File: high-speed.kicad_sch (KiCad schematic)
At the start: 2 parts, among them J301 245863050104829+

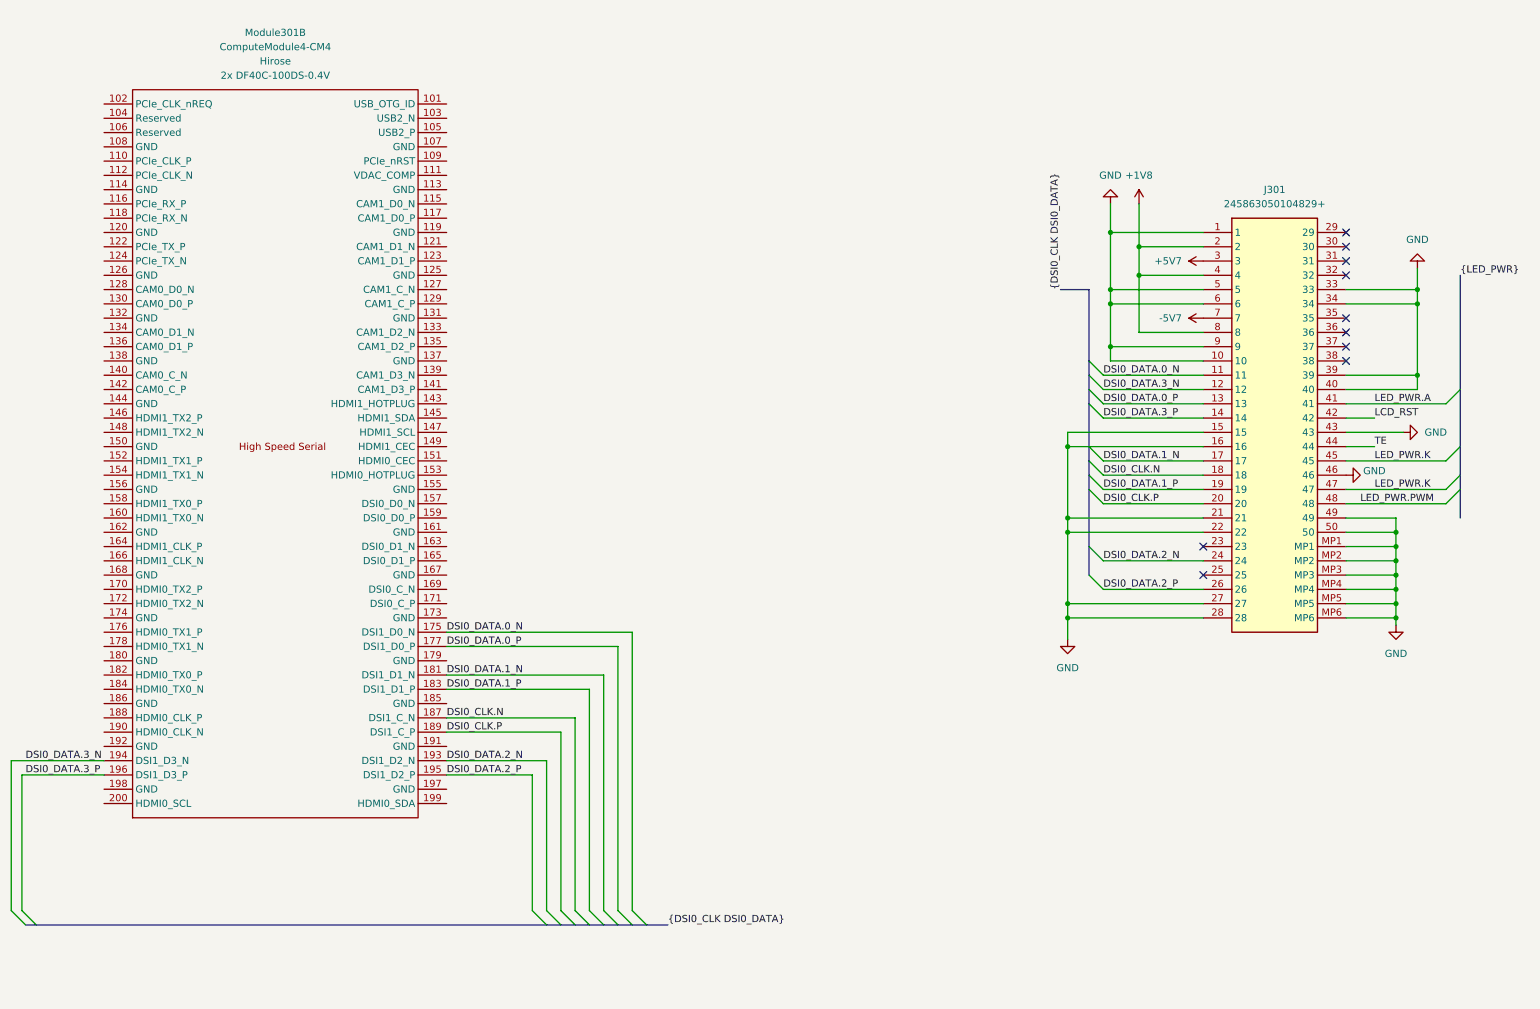
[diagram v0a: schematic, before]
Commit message: more routing
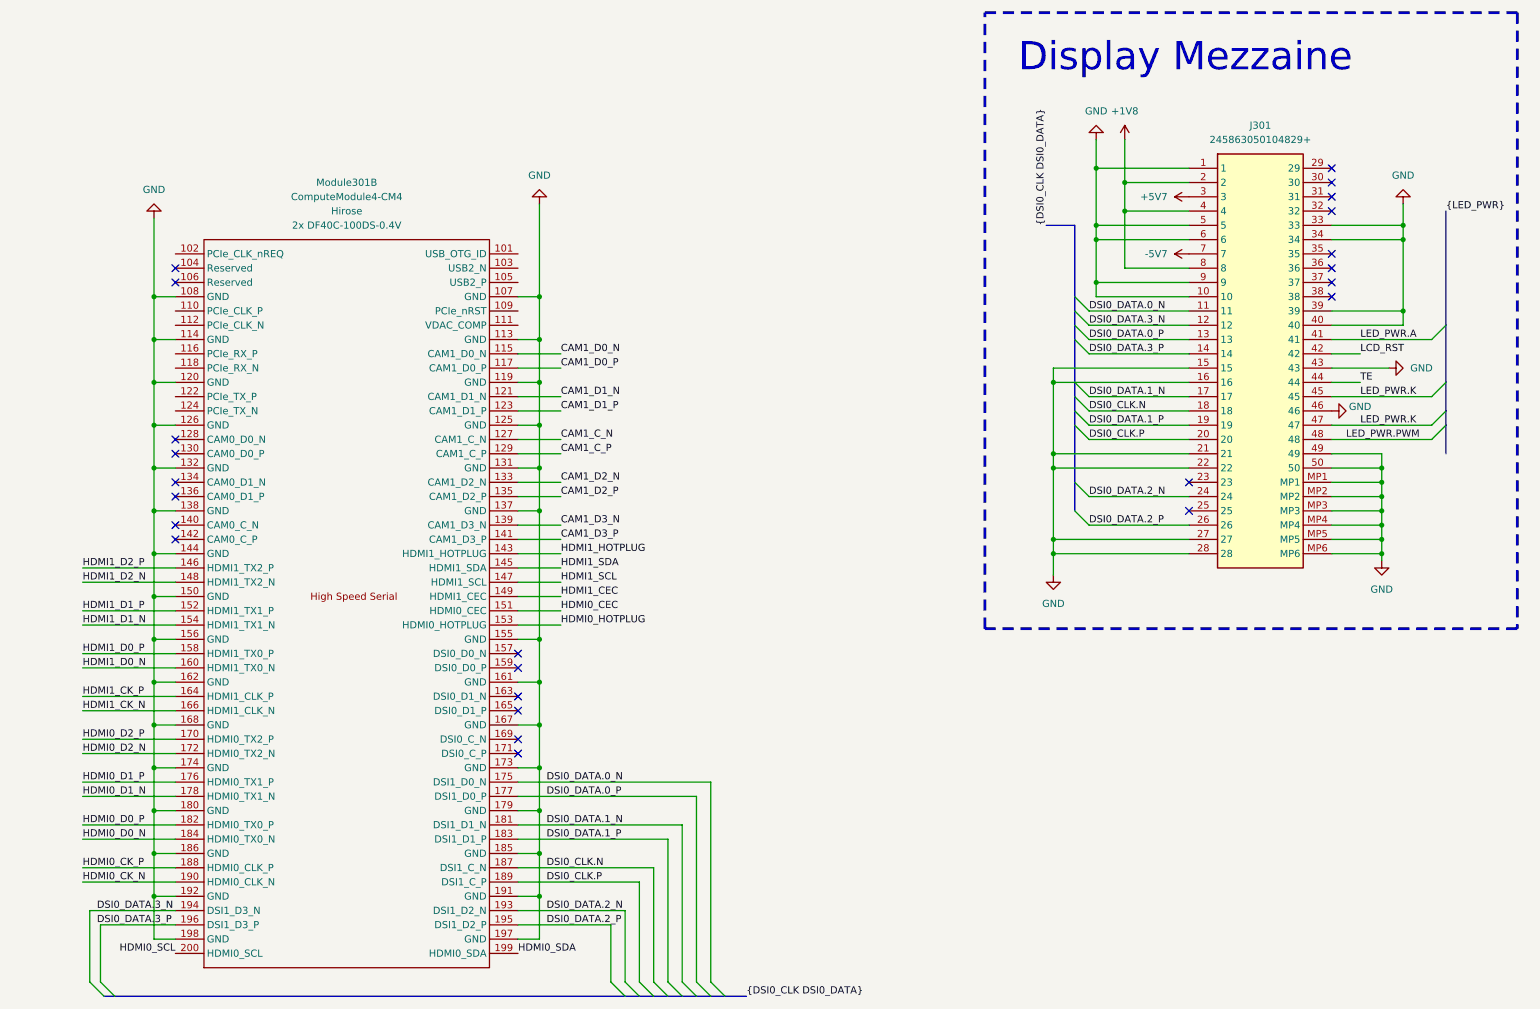
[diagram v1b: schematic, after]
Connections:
- net DSI0_DATA.3_P: no longer Module301.196 (DSI1_D3_P)
- net GND: now also Module301.107 (GND), Module301.108 (GND), Module301.113 (GND), Module301.114 (GND), Module301.119 (GND), Module301.120 (GND), Module301.125 (GND), Module301.126 (GND), Module301.131 (GND), Module301.132 (GND), Module301.137 (GND), Module301.138 (GND), Module301.144 (GND), Module301.150 (GND), Module301.155 (GND), Module301.156 (GND), Module301.161 (GND), Module301.162 (GND), Module301.167 (GND), Module301.168 (GND), Module301.173 (GND), Module301.174 (GND), Module301.179 (GND), Module301.180 (GND), Module301.185 (GND), Module301.186 (GND), Module301.191 (GND), Module301.192 (GND), Module301.197 (GND), Module301.198 (GND)
- net CAM1_D0_N: now reaches Module301.115 (CAM1_D0_N)
- net CAM1_D0_P: now reaches Module301.117 (CAM1_D0_P)
- net CAM1_D1_N: now reaches Module301.121 (CAM1_D1_N)
- net CAM1_D1_P: now reaches Module301.123 (CAM1_D1_P)
- net CAM1_C_N: now reaches Module301.127 (CAM1_C_N)
- net CAM1_C_P: now reaches Module301.129 (CAM1_C_P)
- net CAM1_D2_N: now reaches Module301.133 (CAM1_D2_N)
- net CAM1_D2_P: now reaches Module301.135 (CAM1_D2_P)
- net CAM1_D3_N: now reaches Module301.139 (CAM1_D3_N)
- net CAM1_D3_P: now reaches Module301.141 (CAM1_D3_P)
- net HDMI1_HOTPLUG: now reaches Module301.143 (HDMI1_HOTPLUG)
- net HDMI1_SDA: now reaches Module301.145 (HDMI1_SDA)
- net HDMI1_D2_P: now reaches Module301.146 (HDMI1_TX2_P)
- net HDMI1_SCL: now reaches Module301.147 (HDMI1_SCL)
- net HDMI1_D2_N: now reaches Module301.148 (HDMI1_TX2_N)
- net HDMI1_CEC: now reaches Module301.149 (HDMI1_CEC)
- net HDMI0_CEC: now reaches Module301.151 (HDMI0_CEC)
- net HDMI1_D1_P: now reaches Module301.152 (HDMI1_TX1_P)
- net HDMI0_HOTPLUG: now reaches Module301.153 (HDMI0_HOTPLUG)
- net HDMI1_D1_N: now reaches Module301.154 (HDMI1_TX1_N)
- net HDMI1_D0_P: now reaches Module301.158 (HDMI1_TX0_P)
- net HDMI1_D0_N: now reaches Module301.160 (HDMI1_TX0_N)
- net HDMI1_CK_P: now reaches Module301.164 (HDMI1_CLK_P)
- net HDMI1_CK_N: now reaches Module301.166 (HDMI1_CLK_N)
- net HDMI0_D2_P: now reaches Module301.170 (HDMI0_TX2_P)
- net HDMI0_D2_N: now reaches Module301.172 (HDMI0_TX2_N)
- net HDMI0_D1_P: now reaches Module301.176 (HDMI0_TX1_P)
- net HDMI0_D1_N: now reaches Module301.178 (HDMI0_TX1_N)
- net HDMI0_D0_P: now reaches Module301.182 (HDMI0_TX0_P)
- net HDMI0_D0_N: now reaches Module301.184 (HDMI0_TX0_N)
- net HDMI0_CK_P: now reaches Module301.188 (HDMI0_CLK_P)
- net HDMI0_CK_N: now reaches Module301.190 (HDMI0_CLK_N)
- net HDMI0_SDA: now reaches Module301.199 (HDMI0_SDA)
- net HDMI0_SCL: now reaches Module301.200 (HDMI0_SCL)
- no-connect marks 10 -> 24
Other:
- note added: "Display Mezzaine"
- moved on the sheet: J301, Module301B
